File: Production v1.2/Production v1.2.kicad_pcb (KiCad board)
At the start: 2 copper layers, 35 x 31.2 mm, 55 parts, among them J1 530480510, J2 530480410, J3 USB4085-GF-A_REVB, J4 FH34SRJ-16S-0.5SH_50_, U1 ATSAMD21G18A-AUT, U2 ADR02AUJZ-REEL7, U3 ADR06BUJZ-REEL7, U4 MAX3323EEUE+T, U5 AP7375-33SA-7, Y1 ECS-.327-12.5-1210-TR

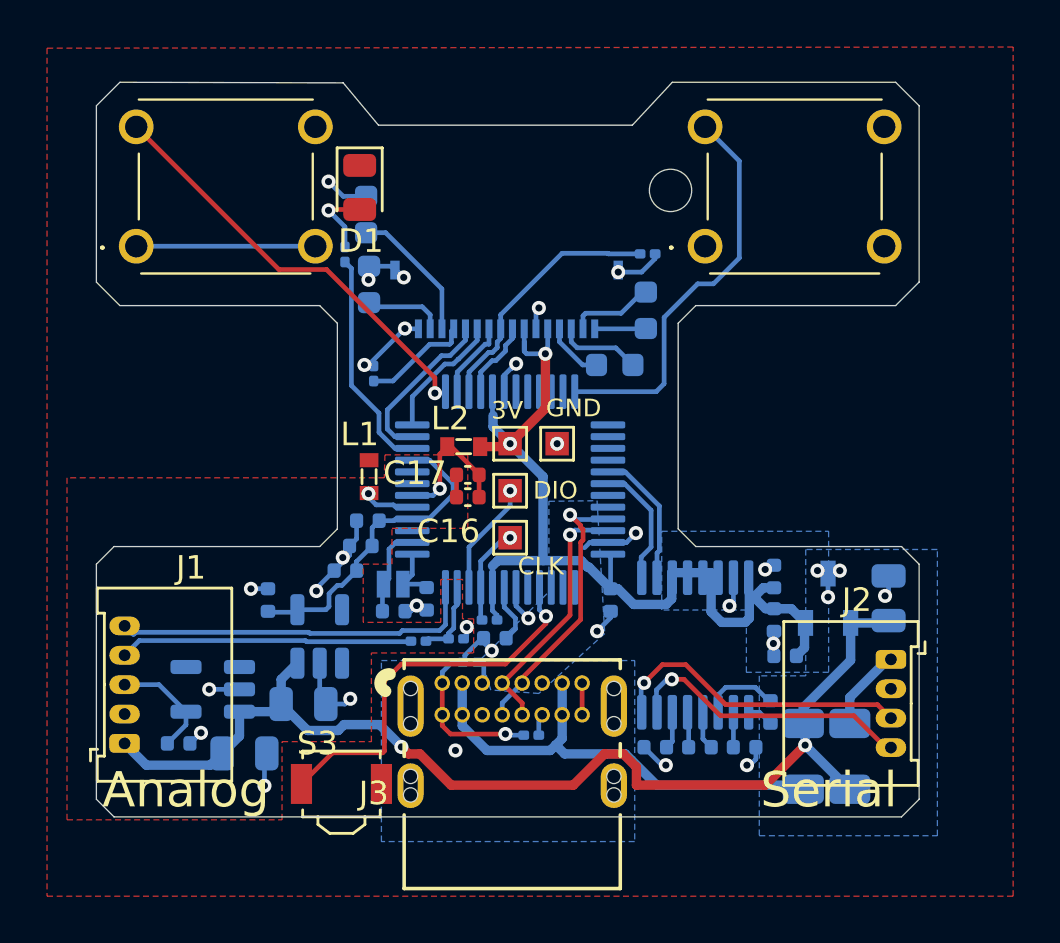
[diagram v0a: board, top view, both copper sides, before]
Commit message: Final tweaks for production v1.2, as manufactured
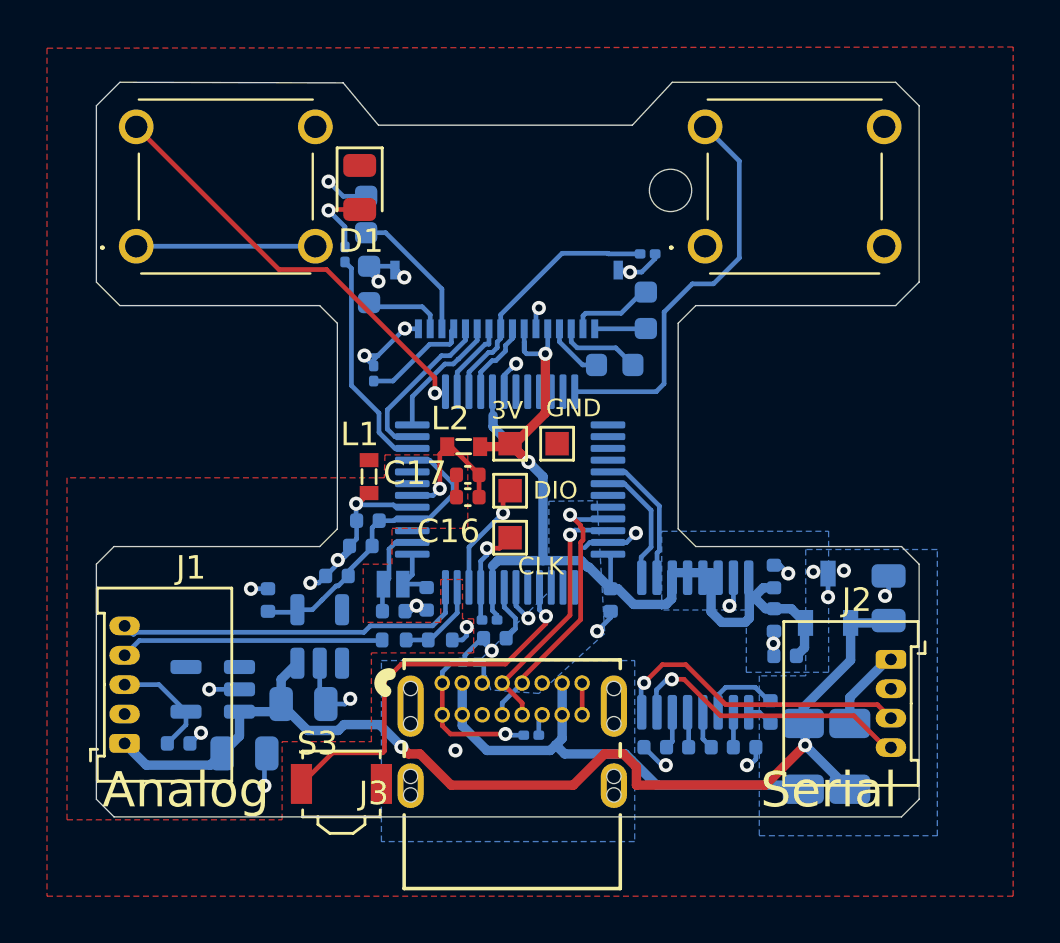
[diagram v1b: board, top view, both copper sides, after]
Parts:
- C13: value 2.2uF,50V+ -> 2.2uF,100V
- C23, C25: value .1uF, 50V -> .1uF, 100V
- L1: value BLM15AX601SN1D -> 600 MHz @ 100 MHz
- L2: value BLM15AX601SN1D -> 600 Ohm @ 100 MHz
- R4, R5: footprint Resistor_SMD:R_0201_0603Metric -> Resistor_SMD:R_0402_1005Metric
- moved R4 1.03 mm to (101.7, 88.2)
- moved R5 0.67 mm to (103.6, 88.2)
- moved C20 0.43 mm to (99.2, 85.5)
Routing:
- net GNDANA: track 15.1 -> 17.5 mm
- net +3V3: track 42.2 -> 44.6 mm
- net GND: track 42.5 -> 44.1 mm, vias 25 -> 24
- net ZOOM: track 12.5 -> 11.2 mm
- net ZSIG: track 3.34 -> 3.91 mm
